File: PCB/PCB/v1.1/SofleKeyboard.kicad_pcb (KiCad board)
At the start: 2 copper layers, 205.9 x 114.2 mm, 203 parts, among them J1 , J10 , J11 , J12 , J13 , J14 , J15 , J16 , J17 , J18 , J19 , J2 , J20 , J21 DATA Port, J22 DATA Port, J23 Conn_01x04, J24 , J25 , J26 , J27 , J28 , J29 , J3 , J30 USB_C_Receptacle_USB2.0, J31 USB_C_Receptacle_USB2.0, J32 , J33 , J4 , J5 , J6 , J7 , J8 , J9 , Q1 AO3407, Q2 AO3407, SW1 1u, SW10 1u, SW11 1u, SW12 1u, SW13 1u, SW14 1u, SW15 1u, SW16 1u, SW17 1u, SW18 1u, SW19 1u, SW2 1u, SW20 1u, SW21 1u, SW22 1u, SW23 1u, SW24 1u, SW25 1u, SW26 1u, SW27 1u, SW28 , SW29 1u, SW3 1u, SW30 1u, SW31 1u, SW32 1u, SW33 1u, SW34 1u, SW35 1u, SW36 1u, SW37 1u, SW38 1u, SW39 1u, SW4 1u, SW40 1u, SW41 1u, SW42 1.5u, SW43 1u, SW44 , SW45 , SW46 RST, SW5 1u, SW6 1u, SW7 1u, SW8 1u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

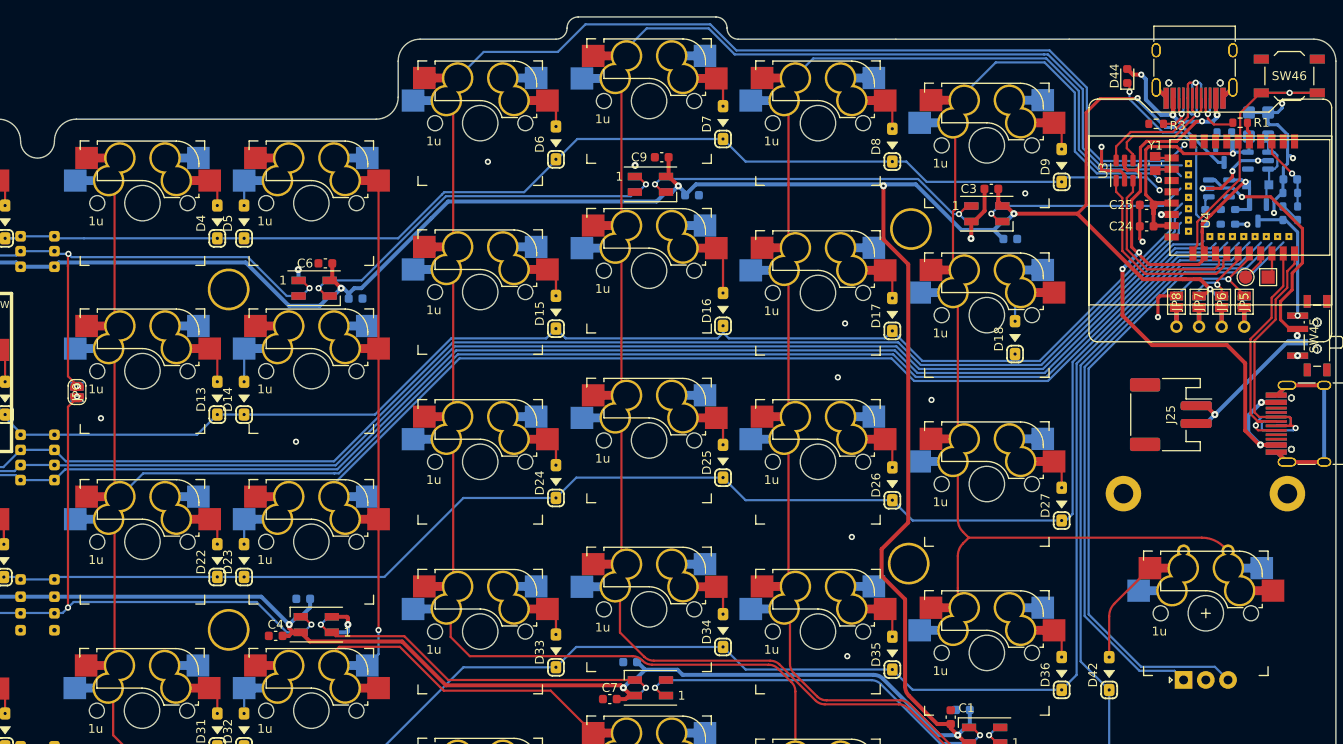
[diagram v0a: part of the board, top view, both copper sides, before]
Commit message: Update PCB
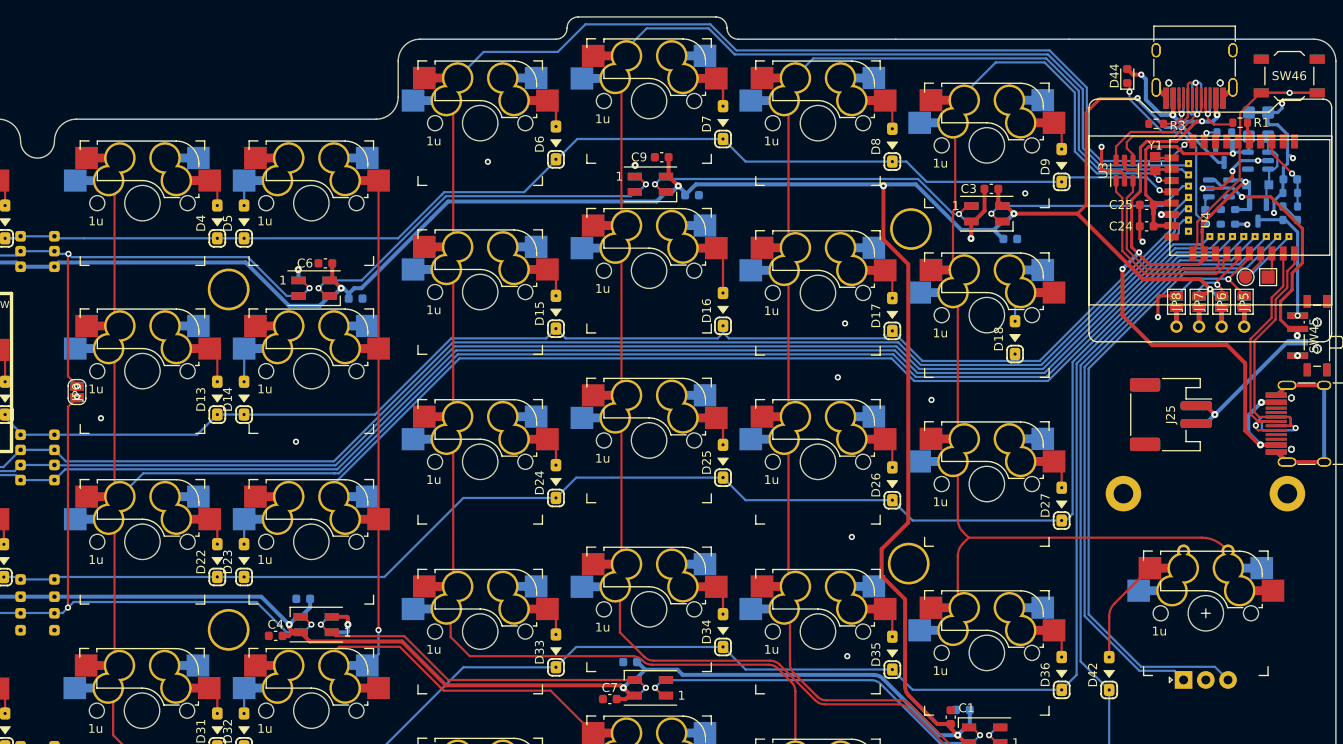
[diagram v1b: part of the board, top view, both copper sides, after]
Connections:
- U4 pad 10: unconnected-(U4-Pad10) -> col2
- U4 pad 12: unconnected-(U4-Pad12) -> col3
- U4 pad 14: unconnected-(U4-Pad14) -> col4
- U4 pad 15: unconnected-(U4-Pad15) -> SW25A
- U4 pad 16: unconnected-(U4-Pad16) -> RGB_BLACKPILL
- U4 pad 17: unconnected-(U4-Pad17) -> row0
- U4 pad 18: unconnected-(U4-Pad18) -> row1
- U4 pad 20: unconnected-(U4-Pad20) -> col1'
- U4 pad 22: unconnected-(U4-Pad22) -> col2'
- U4 pad 28: unconnected-(U4-Pad28) -> col3'
- U4 pad 30: unconnected-(U4-Pad30) -> col0
- U4 pad 32: unconnected-(U4-Pad32) -> col1
- U4 pad 34: unconnected-(U4-Pad34) -> row2
- U4 pad 36: unconnected-(U4-Pad36) -> row3
- U4 pad 38: unconnected-(U4-Pad38) -> row4
- U4 pad 40: unconnected-(U4-Pad40) -> ENCA
- U4 pad 42: unconnected-(U4-Pad42) -> ENCB
- U4 pad 9: unconnected-(U4-Pad9) -> POWER_PIN
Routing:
- net POWER_PIN: track 1.82 -> 4.08 mm, vias 0 -> 1
- net row0: track 200.8 -> 202.2 mm
- net col3': track 226.6 -> 227.7 mm
- net SW25A: track 128.1 -> 129.2 mm
- net col2: track 208.2 -> 209.3 mm
- net col4: track 181.8 -> 182.9 mm
- net col1': track 284.2 -> 285.2 mm
- net ENCA: track 68.9 -> 70.0 mm
- net row1: track 196.2 -> 197.2 mm
- net col0: track 240.1 -> 241.1 mm
- net RGB_BLACKPILL: track 24.1 -> 25.1 mm
- net col2': track 250.0 -> 251.0 mm
- net row4: track 156.5 -> 157.4 mm
- net row2: track 225.9 -> 226.8 mm
- net col1: track 211.2 -> 212.1 mm
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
